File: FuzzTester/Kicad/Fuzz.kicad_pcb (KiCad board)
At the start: 2 copper layers, 180 x 100 mm, 133 parts, among them J1 Audio In/Out JST XH, J10 Key Pad JST XH, J11 1602 LCD JST XH, J2 POT B10K JST XH, J3 POT B5K JST XH, J4 VOL POT A100K JST XH, J5 TestPower_PinHeader, J6 9V Power JST XH, J7 Boot Reset PinHeader, J8 SPI Test PinHeader, J9 SWD_PinHeader, Q1 PN2222A, Q10 2SC1815, Q11 S8050, Q12 S9013, Q13 S9014, Q14 S9018, Q15 BC848B, Q16 2SC1623, Q17 MPSA18, Q18 MPSA18, Q19 2N5088, Q2 MMBT3904, Q20 2N5088, Q21 PN2222A, Q22 MMBT3904, Q23 MMBT5551L, Q24 MMBTA42, Q25 BC807, Q26 BC846, Q27 BC847B, Q28 BC847C, Q29 C945, Q3 MMBT5551L, Q30 2SC1815, Q31 S8050, Q32 S9013, Q33 S9014, Q34 S9018, Q35 BC848B, Q36 2SC1623, Q37 MPSA18, Q38 MPSA18, Q39 2N5088, Q4 MMBTA42, Q40 2N5088, Q5 BC807, Q6 BC846, Q7 BC847B, Q8 BC847C, Q9 C945, U1 AMS1117-5.0, U10 CD4052B, U11 CD4052B, U12 CD4052B, U13 CD4052B, U14 CD4051B, U15 CD4052B, U16 CD4051B, U17 CD4052B, U18 CD4052B, U19 CD4052B, U2 AMS1117-3.3, U20 74HC595, U21 CD4051B, U3 STM32F103C8Tx, U4 CD4051B, U5 74HC595, U6 CD4052B, U7 CD4051B, U8 CD4052B, U9 CD4051B, Y1 8MHz

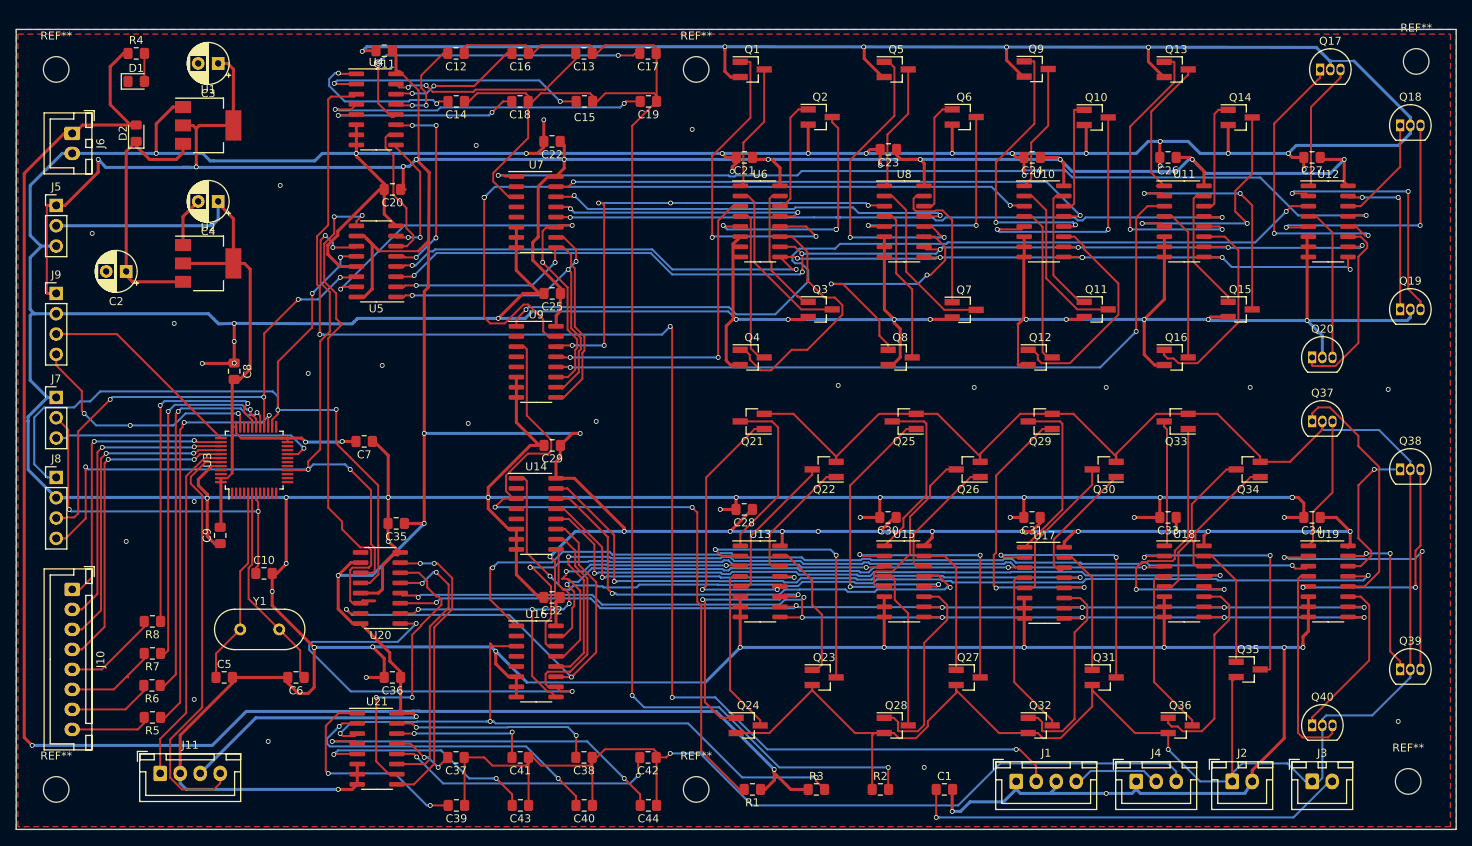
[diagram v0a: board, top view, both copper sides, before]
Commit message: PCB Placement 100x82
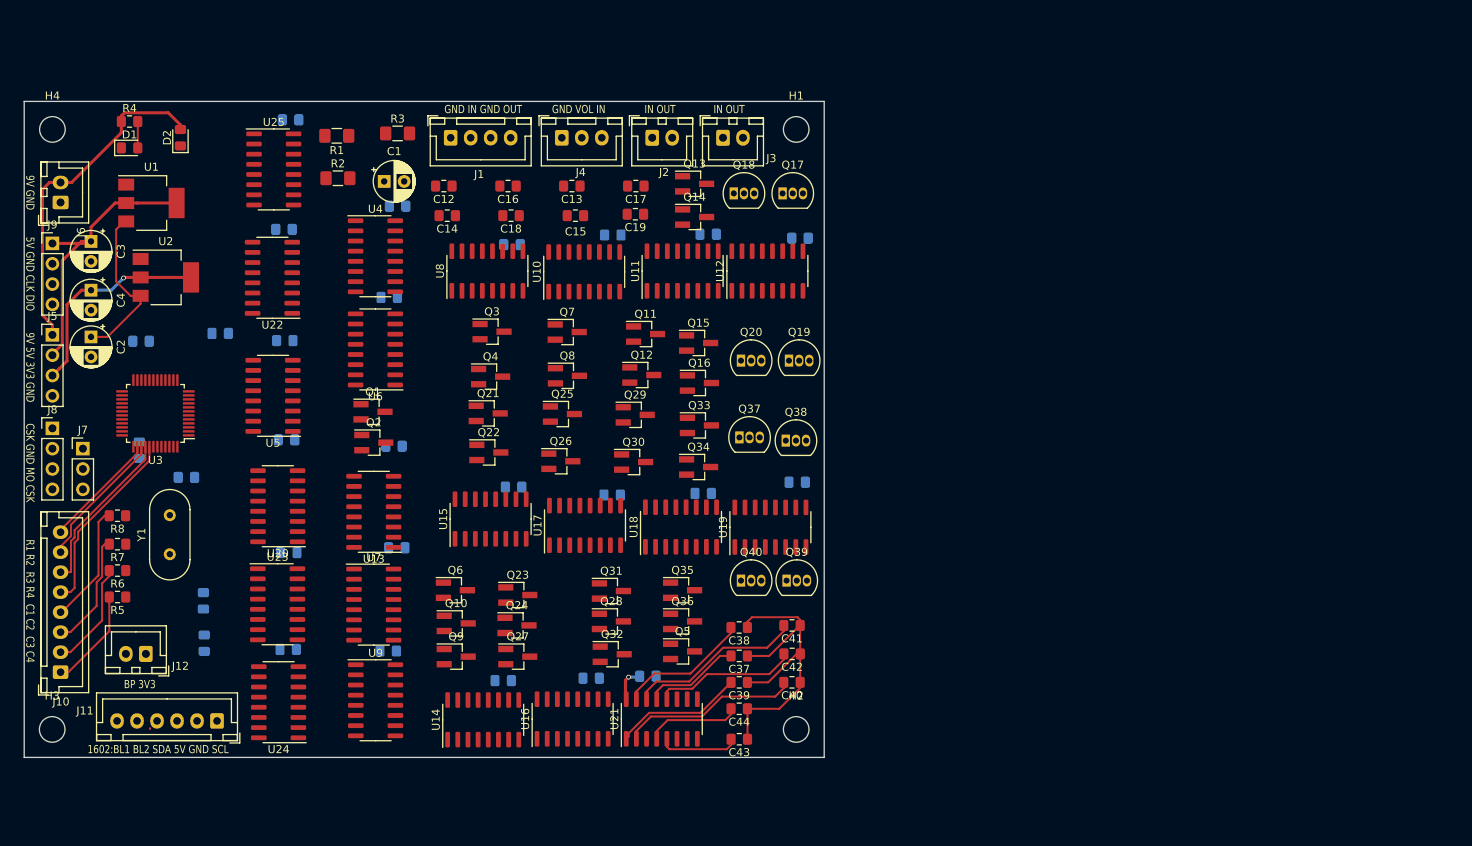
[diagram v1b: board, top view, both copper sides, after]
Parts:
- removed REF** (x6): MountingHole_3.2mm_M3, MountingHole:MountingHole_3.2mm_M3
- added C45: 100nF, Capacitor_SMD:C_0805_2012Metric_Pad1.15x1.40mm_HandSolder, B.Cu at (63.3, 32.3)
- added C46: 100nF, Capacitor_SMD:C_0805_2012Metric_Pad1.15x1.40mm_HandSolder, B.Cu at (63.0, 98.5)
- added C47: 100nF, Capacitor_SMD:C_0805_2012Metric_Pad1.15x1.40mm_HandSolder, B.Cu at (62.5, 46.0)
- added C48: 100nF, Capacitor_SMD:C_0805_2012Metric_Pad1.15x1.40mm_HandSolder, B.Cu at (63.1, 86.4)
- added H1: MountingHole, MountingHole:MountingHole_3.2mm_M3, F.Cu at (126.5, 33.5)
- added H2: MountingHole, MountingHole:MountingHole_3.2mm_M3, F.Cu at (126.5, 108.5)
- added H3: MountingHole, MountingHole:MountingHole_3.2mm_M3, F.Cu at (33.5, 108.5)
- added H4: MountingHole, MountingHole:MountingHole_3.2mm_M3, F.Cu at (33.5, 33.5)
- added J12: Bypass Switch JST XH, Connector_JST:JST_XH_B2B-XH-A_1x02_P2.50mm_Vertical, F.Cu at (45.2, 99.1)
- added U22: 4504, Package_SO:SOIC-16_3.9x9.9mm_P1.27mm, F.Cu at (61.0, 52.0)
- added U23: 4504, Package_SO:SOIC-16_3.9x9.9mm_P1.27mm, F.Cu at (61.7, 92.9)
- added U24: 4504, Package_SO:SOIC-16_3.9x9.9mm_P1.27mm, F.Cu at (61.8, 105.1)
- added U25: CD4053B, Package_SO:SOIC-16_3.9x9.9mm_P1.27mm, F.Cu at (61.2, 38.5)
- C1: footprint Capacitor_SMD:C_0805_2012Metric_Pad1.15x1.40mm_HandSolder -> Capacitor_THT:CP_Radial_D5.0mm_P2.50mm
- C10, C11, C20, C21, C22, C23, C24, C25, C26, C27, C28, C29, C30, C31, C32, C33, C34, C35, C36, C5, C6, C7, C8, C9: moved to B.Cu
- J11: value 1602 LCD JST XH -> LCD JST XH; footprint Connector_JST:JST_XH_B4B-XH-A_1x04_P2.50mm_Vertical -> Connector_JST:JST_XH_B6B-XH-A_1x06_P2.50mm_Vertical
- J5: value TestPower_PinHeader -> PowerTest_PinHeader; footprint Connector_PinHeader_2.54mm:PinHeader_1x03_P2.54mm_Vertical -> Connector_PinHeader_2.54mm:PinHeader_1x04_P2.54mm_Vertical
- R1, R2, R3: footprint Resistor_SMD:R_0805_2012Metric_Pad1.15x1.40mm_HandSolder -> Resistor_SMD:R_1206_3216Metric_Pad1.42x1.75mm_HandSolder
- moved J3 109.1 mm to (117.3, 34.5)
- moved J2 108.3 mm to (108.5, 34.5)
- moved J4 107.8 mm to (97.2, 34.5)
- moved J1 107.1 mm to (83.3, 34.5)
- moved C1 103.3 mm to (75.0, 40.0)
- moved Q9 103.2 mm to (84.0, 99.4)
- moved R2 102.2 mm to (69.2, 39.6)
- moved Q10 102.0 mm to (84.0, 95.2)
- moved R3 97.3 mm to (76.7, 34.0)
- moved R1 96.8 mm to (69.1, 34.3)
- moved Q6 86.9 mm to (83.9, 91.1)
- moved Q18 83.7 mm to (118.7, 41.5)
- moved Q39 77.5 mm to (125.3, 89.9)
- moved Q5 77.5 mm to (112.3, 98.8)
- moved Q38 76.9 mm to (125.2, 72.4)
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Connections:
- C11 pad 1: +5V -> +9V
- C20 pad 1: +5V -> +3V3
- C21 pad 1: +5V -> +9V
- C22 pad 1: +5V -> +9V
- C23 pad 1: +5V -> +9V
- C24 pad 1: +5V -> +9V
- C25 pad 1: +5V -> +9V
- C26 pad 1: +5V -> +9V
- C27 pad 1: +5V -> +9V
- C28 pad 1: +5V -> +9V
- C29 pad 1: +5V -> +9V
- C30 pad 1: +5V -> +9V
- C31 pad 1: +5V -> +9V
- C32 pad 1: +5V -> +9V
- C33 pad 1: +5V -> +9V
- C34 pad 1: +5V -> +9V
- C35 pad 1: +5V -> +3V3
- C36 pad 1: +5V -> +9V
- J1 pad 2: /JACK_IN_SIGNAL -> /AudioInOut/JACK_IN_SIGNAL
- J1 pad 4: /JACK_OUT_SIGNAL -> /AudioInOut/JACK_OUT_SIGNAL
- J10 pad 1: /Mcu/GPIO_KEYPAD_ROW_1 -> Net-(J10-Pad1)
- J10 pad 2: /Mcu/GPIO_KEYPAD_ROW_2 -> Net-(J10-Pad2)
- J10 pad 3: /Mcu/GPIO_KEYPAD_ROW_3 -> Net-(J10-Pad3)
- J10 pad 4: /Mcu/GPIO_KEYPAD_ROW_4 -> Net-(J10-Pad4)
- J10 pad 5: Net-(J10-Pad5) -> /Mcu/GPIO_KEYPAD_ROW_4
- J10 pad 6: Net-(J10-Pad6) -> /Mcu/GPIO_KEYPAD_ROW_3
- J10 pad 7: Net-(J10-Pad7) -> /Mcu/GPIO_KEYPAD_ROW_2
- J10 pad 8: Net-(J10-Pad8) -> /Mcu/GPIO_KEYPAD_ROW_1
- J4 pad 2: /JACK_OUT_SIGNAL -> /JACK_OUT_SIGNAL_FROM_FUZZ
- J5 pad 1: +5V -> +9V
- J5 pad 2: +3V3 -> +5V
- J5 pad 3: GND -> +3V3
- J6 pad 1: +9V -> GND
- J6 pad 2: GND -> +9V
- R5 pad 1: /Mcu/GPIO_KEYPAD_COLUMN_4 -> /Mcu/GPIO_KEYPAD_COLUMN_1
- R5 pad 2: Net-(R5-Pad2) -> Net-(J10-Pad1)
- R6 pad 1: /Mcu/GPIO_KEYPAD_COLUMN_3 -> /Mcu/GPIO_KEYPAD_COLUMN_2
- R6 pad 2: Net-(J10-Pad7) -> Net-(J10-Pad2)
- R7 pad 1: /Mcu/GPIO_KEYPAD_COLUMN_2 -> /Mcu/GPIO_KEYPAD_COLUMN_3
- R7 pad 2: Net-(J10-Pad6) -> Net-(J10-Pad3)
- R8 pad 1: /Mcu/GPIO_KEYPAD_COLUMN_1 -> /Mcu/GPIO_KEYPAD_COLUMN_4
- R8 pad 2: Net-(J10-Pad5) -> Net-(J10-Pad4)
- U10 pad 16: +5V -> +9V
- U11 pad 16: +5V -> +9V
- U12 pad 16: +5V -> +9V
- U13 pad 16: +5V -> +9V
- U14 pad 16: +5V -> +9V
- U15 pad 16: +5V -> +9V
- U16 pad 16: +5V -> +9V
- U17 pad 16: +5V -> +9V
- U18 pad 16: +5V -> +9V
- U19 pad 16: +5V -> +9V
- U20 pad 1: /TRANSISTOR_C_GROUP_SELECTION_1 -> /TRANSISTOR_C_GROUP_SELECTION_3V3_1
- U20 pad 15: /TRANSISTOR_C_GROUP_SELECTION_0 -> /TRANSISTOR_C_GROUP_SELECTION_3V3_0
- U20 pad 16: +5V -> +3V3
- U20 pad 2: /TRANSISTOR_C_GROUP_SELECTION_2 -> /TRANSISTOR_C_GROUP_SELECTION_3V3_2
- U20 pad 3: /TRANSISTOR_C_SELECTION_0 -> /TRANSISTOR_C_SELECTION_3V3_0
- U20 pad 4: /TRANSISTOR_C_SELECTION_1 -> /TRANSISTOR_C_SELECTION_3V3_1
- U20 pad 5: /CAPACITOR_D_SELECTION_0 -> /CAPACITOR_D_SELECTION_3V3_0
- U20 pad 6: /CAPACITOR_D_SELECTION_1 -> /CAPACITOR_D_SELECTION_3V3_1
- U20 pad 7: /CAPACITOR_D_SELECTION_2 -> /CAPACITOR_D_SELECTION_3V3_2
- U21 pad 16: +5V -> +9V
- U3 pad 12: Net-(U3-Pad12) -> /Mcu/BYPASS_SWITCH_3V3
- U3 pad 13: Net-(U3-Pad13) -> /BYPASS_MODE_3V3
- U4 pad 16: +5V -> +9V
- U4 pad 3: /JACK_IN_SIGNAL -> /JACK_IN_SIGNAL_THROUGH_FUZZ
- U5 pad 1: /TRANSISTOR_B_GROUP_SELECTION_1 -> /TRANSISTOR_B_GROUP_SELECTION_3V3_1
- U5 pad 15: /TRANSISTOR_B_GROUP_SELECTION_0 -> /TRANSISTOR_B_GROUP_SELECTION_3V3_0
- U5 pad 16: +5V -> +3V3
- U5 pad 2: /TRANSISTOR_B_GROUP_SELECTION_2 -> /TRANSISTOR_B_GROUP_SELECTION_3V3_2
- U5 pad 3: /TRANSISTOR_B_SELECTION_0 -> /TRANSISTOR_B_SELECTION_3V3_0
- U5 pad 4: /TRANSISTOR_B_SELECTION_1 -> /TRANSISTOR_B_SELECTION_3V3_1
- U5 pad 5: /CAPACITOR_A_SELECTION_0 -> /CAPACITOR_A_SELECTION_3V3_0
- U5 pad 6: /CAPACITOR_A_SELECTION_1 -> /CAPACITOR_A_SELECTION_3V3_1
- U5 pad 7: /CAPACITOR_A_SELECTION_2 -> /CAPACITOR_A_SELECTION_3V3_2
- U6 pad 16: +5V -> +9V
- U7 pad 16: +5V -> +9V
- U8 pad 16: +5V -> +9V
- U9 pad 16: +5V -> +9V
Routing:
- net GND: track 1339.9 -> 0.00 mm, vias 89 -> 0
- net +5V: track 598.5 -> 35.6 mm, vias 27 -> 0
- net /TransistorsC/EMITTER: track 272.7 -> 0.00 mm, vias 1 -> 0
- net /TransistorsB/BASE: track 191.5 -> 0.00 mm, vias 2 -> 0
- net /JACK_IN_SIGNAL: track 175.6 -> 0.00 mm, vias 4 -> 0
- net +9V: track 207.4 -> 46.7 mm, vias 2 -> 1
- net /TRANSISTOR_B_SELECTION_0: track 138.3 -> 0.00 mm, vias 7 -> 0
- net /TRANSISTOR_C_SELECTION_1: track 136.6 -> 0.00 mm, vias 7 -> 0
- net /TRANSISTOR_B_SELECTION_1: track 135.0 -> 0.00 mm, vias 8 -> 0
- net /TRANSISTOR_C_SELECTION_0: track 132.8 -> 0.00 mm, vias 6 -> 0
- net /TransistorsC/TG_5_BASE: track 121.9 -> 0.00 mm, vias 2 -> 0
- net /TransistorsB/TG_5_BASE: track 115.8 -> 0.00 mm, vias 2 -> 0
- net /TransistorsC/TG_5_COLLECTOR: track 113.5 -> 0.00 mm, vias 2 -> 0
- net /TransistorsB/TG_5_COLLECTOR: track 111.6 -> 0.00 mm, vias 2 -> 0
- net /SPI2_CSK: track 102.5 -> 0.00 mm, vias 4 -> 0
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- removed copper zone on B.Cu, net GND
- removed copper zone on F.Cu, net GND
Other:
- board size 180 x 100 mm -> 100 x 82 mm
- board text added: "1602:BL1 BL2 SDA 5V GND SCL"
- board text added: "5V GND CLK DIO"
- board text added: "9V 5V 3V3 GND"
- board text added: "9V GND"
- board text added: "BP 3V3"
- board text added: "CSK GND MO CSK"
- board text added: "GND IN GND OUT"
- board text added: "GND VOL IN"
- board text added: "IN OUT"
- board text added: "R1 R2 R3 R4 C1 C2 C3 C4"

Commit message: Starting to route
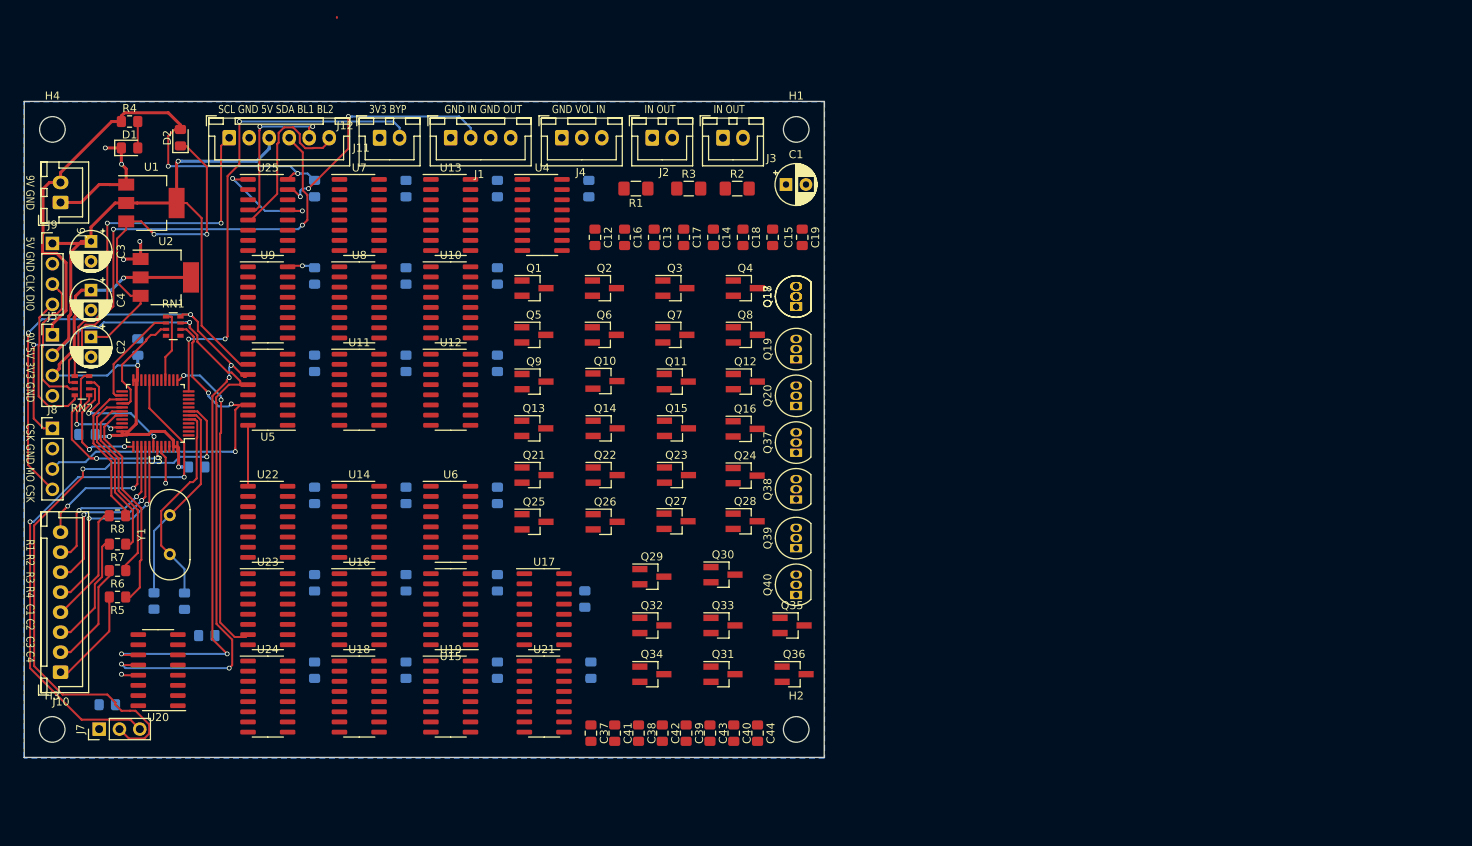
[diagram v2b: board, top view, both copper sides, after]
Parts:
- added RN1: R_Pack04, Resistor_SMD:R_Array_Convex_4x0603, F.Cu at (48.6, 58.1)
- added RN2: R_Pack04, Resistor_SMD:R_Array_Convex_4x0603, F.Cu at (37.2, 65.5)
- moved J11 72.9 mm to (55.6, 34.5), turned to 0 degrees
- moved J12 70.8 mm to (74.4, 34.5), turned to 0 degrees
- moved U9 51.5 mm to (60.5, 55.1)
- moved C1 50.2 mm to (125.2, 40.4)
- moved R2 49.9 mm to (119.1, 40.9)
- moved U7 48.7 mm to (71.9, 44.2)
- moved C25 47.8 mm to (66.3, 51.8), turned to 270 degrees
- moved U18 45.5 mm to (71.9, 104.4), turned to 0 degrees
- moved U19 45.2 mm to (83.3, 104.4), turned to 0 degrees
- moved C22 44.9 mm to (77.7, 40.9), turned to 270 degrees
- moved C34 44.2 mm to (89.2, 101.1), turned to 270 degrees
- moved Q5 43.7 mm to (93.7, 59.2)
- moved C33 43.2 mm to (77.7, 101.1), turned to 270 degrees
- moved U11 43.1 mm to (71.9, 66.0), turned to 0 degrees
- moved U12 42.3 mm to (83.3, 66.0), turned to 0 degrees
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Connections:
- U3 pad 16: /GPIO_LATCH -> /Mcu/GPIO_LATCH_MCU
- U3 pad 26: /SPI2_CSK -> /Mcu/SPI2_CSK_MCU
- U3 pad 28: /SPI2_MOSI -> /Mcu/SPI2_MOSI_MCU
- U3 pad 34: /Mcu/SYS_JTMS_SWDIO -> /Mcu/SYS_JTMS_SWDIO_MCU
- U3 pad 37: /Mcu/SYS_JTICK_SWCLK -> /Mcu/SYS_JTICK_SWCLK_MCU
- U3 pad 42: /Mcu/I2C1_SCL -> /Mcu/I2C1_SCL_MCU
- U3 pad 43: /Mcu/I2C1_SDA -> /Mcu/I2C1_SDA_MCU
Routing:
- net /GPIO_LATCH: track 0.00 -> 107.8 mm, vias 0 -> 6
- net /SPI2_CSK: track 0.00 -> 99.9 mm, vias 0 -> 4
- net /Mcu/NRST: track 0.00 -> 73.7 mm, vias 0 -> 2
- net /Mcu/PB2: track 0.00 -> 70.7 mm, vias 0 -> 2
- net /Mcu/BYPASS_SWITCH_3V3: track 0.00 -> 60.6 mm, vias 0 -> 3
- net /Mcu/I2C1_SDA: track 0.00 -> 57.0 mm, vias 0 -> 2
- net /Mcu/I2C1_SCL: track 0.00 -> 48.6 mm, vias 0 -> 2
- net /SPI2_MOSI: track 0.00 -> 47.2 mm, vias 0 -> 3
- net +3V3: track 26.6 -> 72.4 mm, vias 1 -> 4
- net /CapacitorsD/CAPACITOR_AUDIO_OUTPUT: track 43.9 -> 0.00 mm
- net +5V: track 35.6 -> 79.4 mm, vias 0 -> 1
- net /BYPASS_MODE_3V3: track 0.00 -> 39.4 mm, vias 0 -> 2
- net /AudioInOut/JACK_IN_SIGNAL: track 0.00 -> 32.0 mm, vias 0 -> 3
- net +9V: track 46.7 -> 74.1 mm, vias 1 -> 3
- net GND: track 0.00 -> 27.3 mm, vias 0 -> 6
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- added copper zone on B.Cu, net GND
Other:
- board text added: "3V3 BYP"
- board text added: "SCL GND 5V SDA BL1 BL2"
- board text removed: "1602:BL1 BL2 SDA 5V GND SCL"
- board text removed: "BP 3V3"
